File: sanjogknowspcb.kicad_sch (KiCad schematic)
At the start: 12 parts, among them SW1 SW_Push

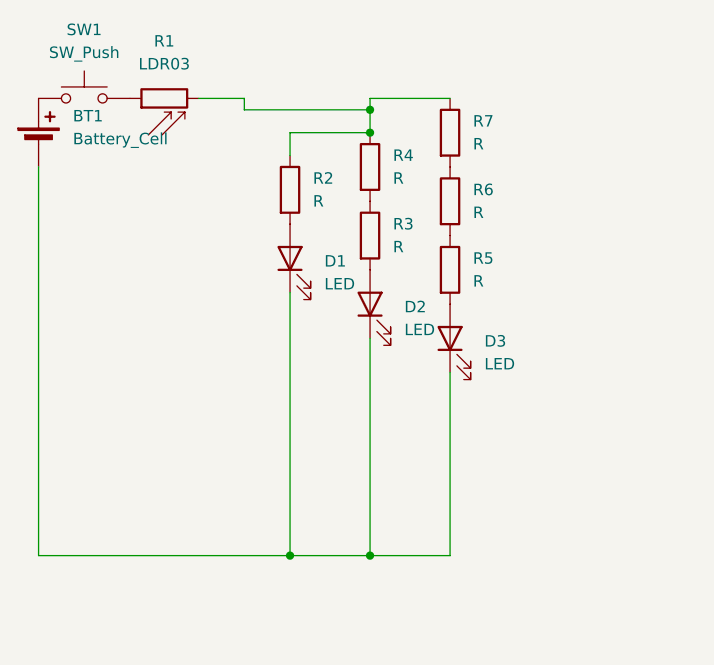
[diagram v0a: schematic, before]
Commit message: Add files via upload
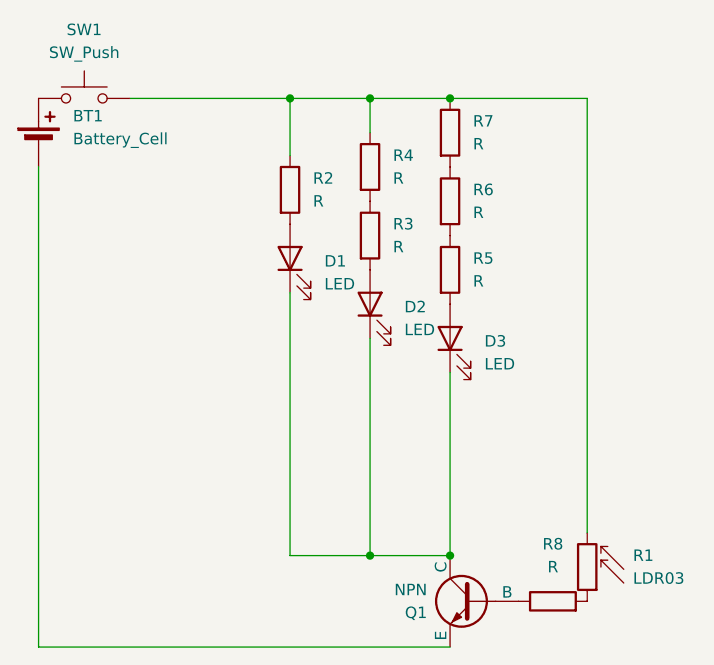
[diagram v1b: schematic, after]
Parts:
- added Q1: NPN, Package_TO_SOT_THT:TO-92L_HandSolder, symbol Simulation_SPICE:NPN
- added R8: R, Resistor_THT:R_Axial_DIN0207_L6.3mm_D2.5mm_P7.62mm_Horizontal, symbol Device:R
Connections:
- net at D1.1 (K), D2.1 (K), D3.1 (K): now also Q1.1 (C); no longer BT1.2 (-)
- net at R1.2, R2.1, R4.1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: now also SW1.2
- net at R1.1: now also R8.2; no longer SW1.2
- new net: Q1.2 (B), R8.1
- new net: BT1.2 (-), Q1.3 (E)
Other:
- moved on the sheet: R1
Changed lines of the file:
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@@
 	(paper "A4")
-	(junction
-		(at 66.04 124.46)
-		(diameter 0)
-		(color 0 0 0 0)
-	)
-	(junction
-		(at 74.93 77.47)
-		(diameter 0)
-		(color 0 0 0 0)
-	)
 	(junction
 		(at 74.93 124.46)
@@
 	)
 	(junction
-		(at 74.93 74.93)
+		(at 83.82 73.66)
 		(diameter 0)
 		(color 0 0 0 0)
 	)
-	(wire
-		(pts
-			(xy 66.04 80.01) (xy 66.04 77.47)
-		)
-		(stroke
-			(width 0)
-			(type default)
-		)
-	)
-	(wire
-		(pts
-			(xy 74.93 73.66) (xy 83.82 73.66)
-		)
-		(stroke
-			(width 0)
-			(type default)
-		)
-	)
-	(wire
-		(pts
-			(xy 74.93 77.47) (xy 74.93 74.93)
-		)
-		(stroke
-			(width 0)
-			(type default)
-		)
-	)
-	(wire
-		(pts
-			(xy 60.96 73.66) (xy 60.96 74.93)
-		)
-		(stroke
-			(width 0)
-			(type default)
-		)
-	)
-	(wire
-		(pts
-			(xy 74.93 74.93) (xy 60.96 74.93)
-		)
-		(stroke
-			(width 0)
-			(type default)
-		)
-	)
-	(wire
-		(pts
-			(xy 55.88 73.66) (xy 60.96 73.66)
-		)
-		(stroke
-			(width 0)
-			(type default)
-		)
-	)
-	(wire
-		(pts
-			(xy 38.1 124.46) (xy 38.1 81.28)
-		)
-		(stroke
-			(width 0)
-			(type default)
-		)
-	)
-	(wire
-		(pts
-			(xy 66.04 77.47) (xy 74.93 77.47)
-		)
-		(stroke
-			(width 0)
-			(type default)
-		)
-	)
-	(wire
-		(pts
-			(xy 74.93 74.93) (xy 74.93 73.66)
+	(junction
+		(at 66.04 73.66)
+		(diameter 0)
+		(color 0 0 0 0)
+	)
+	(junction
+		(at 83.82 124.46)
+		(diameter 0)
+		(color 0 0 0 0)
+	)
+	(junction
+		(at 74.93 73.66)
+		(diameter 0)
+		(color 0 0 0 0)
+	)
+	(wire
+		(pts
+			(xy 66.04 73.66) (xy 66.04 80.01)
+		)
+		(stroke
+			(width 0)
+			(type default)
+		)
+	)
+	(wire
+		(pts
+			(xy 74.93 73.66) (xy 74.93 77.47)
+		)
+		(stroke
+			(width 0)
+			(type default)
+		)
+	)
+	(wire
+		(pts
+			(xy 83.82 104.14) (xy 83.82 124.46)
+		)
+		(stroke
+			(width 0)
+			(type default)
+		)
+	)
+	(wire
+		(pts
+			(xy 99.06 73.66) (xy 83.82 73.66)
+		)
+		(stroke
+			(width 0)
+			(type default)
+		)
+	)
+	(wire
+		(pts
+			(xy 83.82 73.66) (xy 74.93 73.66)
+		)
+		(stroke
+			(width 0)
+			(type default)
+		)
+	)
+	(wire
+		(pts
+			(xy 99.06 121.92) (xy 99.06 73.66)
+		)
+		(stroke
+			(width 0)
+			(type default)
+		)
+	)
+	(wire
+		(pts
+			(xy 74.93 73.66) (xy 66.04 73.66)
+		)
+		(stroke
+			(width 0)
+			(type default)
+		)
+	)
+	(wire
+		(pts
+			(xy 83.82 134.62) (xy 38.1 134.62)
+		)
+		(stroke
+			(width 0)
+			(type default)
+		)
+	)
+	(wire
+		(pts
+			(xy 38.1 81.28) (xy 38.1 134.62)
 		)
 		(stroke
@@
 	(wire
 		(pts
-			(xy 38.1 124.46) (xy 66.04 124.46)
-		)
-		(stroke
-			(width 0)
-			(type default)
-		)
-	)
-	(wire
-		(pts
 			(xy 74.93 100.33) (xy 74.93 124.46)
 		)
@@
 	(wire
 		(pts
-			(xy 83.82 104.14) (xy 83.82 124.46)
-		)
-		(stroke
-			(width 0)
-			(type default)
-		)
-	)
-	(wire
-		(pts
 			(xy 66.04 124.46) (xy 74.93 124.46)
 		)
@@
 		(pts
 			(xy 74.93 124.46) (xy 83.82 124.46)
+		)
+		(stroke
+			(width 0)
+			(type default)
+		)
+	)
+	(wire
+		(pts
+			(xy 66.04 73.66) (xy 48.26 73.66)
 		)
 		(stroke
@@
 	)
 	(symbol
+		(lib_id "Simulation_SPICE:NPN")
+		(at 86.36 129.54 0)
+		(mirror y)
+		(unit 1)
+		(exclude_from_sim no)
+		(in_bom yes)
+		(on_board yes)
+		(dnp no)
+		(property "Reference" "Q1"
+			(at 81.28 130.8101 0)
+			(effects
+				(font
+					(size 1.27 1.27)
+				)
+				(justify left)
+			)
+		)
+		(property "Value" "NPN"
+			(at 81.28 128.2701 0)
+			(effects
+				(font
+					(size 1.27 1.27)
+				)
+				(justify left)
+			)
+		)
+		(property "Footprint" "Package_TO_SOT_THT:TO-92L_HandSolder"
+			(at 22.86 129.54 0)
+			(effects
+				(font
+					(size 1.27 1.27)
+				)
+				(hide yes)
+			)
+		)
+		(property "Datasheet" "https://ngspice.sourceforge.io/docs/ngspice-html-manual/manual.xhtml#cha_BJTs"
+			(at 22.86 129.54 0)
+			(effects
+				(font
+					(size 1.27 1.27)
+				)
+				(hide yes)
+			)
+		)
+		(property "Description" "Bipolar transistor symbol for simulation only, substrate tied to the emitter"
+			(at 86.36 129.54 0)
+			(effects
+				(font
+					(size 1.27 1.27)
+				)
+				(hide yes)
+			)
+		)
+		(property "Sim.Device" "NPN"
+			(at 86.36 129.54 0)
+			(effects
+				(font
+					(size 1.27 1.27)
+				)
+				(hide yes)
+			)
+		)
+		(property "Sim.Type" "GUMMELPOON"
+			(at 86.36 129.54 0)
+			(effects
+				(font
+					(size 1.27 1.27)
+				)
+				(hide yes)
+			)
+		)
+		(property "Sim.Pins" "1=C 2=B 3=E"
+			(at 86.36 129.54 0)
+			(effects
+				(font
+					(size 1.27 1.27)
+				)
+				(hide yes)
+			)
+		)
+		(pin "3"
+		)
+		(pin "1"
+		)
+		(pin "2"
+		)
+		(instances
+			(project ""
+				(path "/80278f69-b966-473c-8055-8c9a8f6f86ca"
+					(reference "Q1")
+					(unit 1)
+				)
+			)
+		)
+	)
+	(symbol
 		(lib_id "Device:Battery_Cell")
 		(at 38.1 78.74 0)
@@
 	(symbol
 		(lib_id "Sensor_Optical:LDR03")
-		(at 52.07 73.66 90)
+		(at 99.06 125.73 180)
 		(unit 1)
 		(exclude_from_sim no)
@@
 		(fields_autoplaced yes)
 		(property "Reference" "R1"
-			(at 52.07 67.31 90)
-			(effects
-				(font
-					(size 1.27 1.27)
-				)
+			(at 104.14 124.4599 0)
+			(effects
+				(font
+					(size 1.27 1.27)
+				)
+				(justify right)
 			)
 		)
 		(property "Value" "LDR03"
-			(at 52.07 69.85 90)
-			(effects
-				(font
-					(size 1.27 1.27)
-				)
+			(at 104.14 126.9999 0)
+			(effects
+				(font
+					(size 1.27 1.27)
+				)
+				(justify right)
 			)
 		)
 		(property "Footprint" "OptoDevice:R_LDR_5.1x4.3mm_P3.4mm_Vertical"
-			(at 52.07 69.215 90)
+			(at 94.615 125.73 90)
 			(effects
 				(font
@@
 		)
 		(property "Datasheet" "http://www.elektronica-componenten.nl/WebRoot/StoreNL/Shops/61422969/54F1/BA0C/C664/31B9/2173/C0A8/2AB9/2AEF/LDR03IMP.pdf"
-			(at 53.34 73.66 0)
+			(at 99.06 124.46 0)
 			(effects
 				(font
@@
 		)
 		(property "Description" "light dependent resistor"
-			(at 52.07 73.66 0)
+			(at 99.06 125.73 0)
 			(effects
 				(font
@@
 					(unit 1)
 				)
+			)
+		)
+	)
+	(symbol
+		(lib_id "Device:R")
+		(at 95.25 129.54 90)
+		(unit 1)
+		(exclude_from_sim no)
+		(in_bom yes)
+		(on_board yes)
+		(dnp no)
+		(fields_autoplaced yes)
+		(property "Reference" "R8"
+			(at 95.25 123.19 90)
+			(effects
+				(font
+					(size 1.27 1.27)
+				)
+			)
+		)
+		(property "Value" "R"
+			(at 95.25 125.73 90)
+			(effects
+				(font
+					(size 1.27 1.27)
+				)
+			)
+		)
+		(property "Footprint" "Resistor_THT:R_Axial_DIN0207_L6.3mm_D2.5mm_P7.62mm_Horizontal"
+			(at 95.25 131.318 90)
+			(effects
+				(font
+					(size 1.27 1.27)
+				)
+				(hide yes)
+			)
+		)
+		(property "Datasheet" "~"
+			(at 95.25 129.54 0)
+			(effects
+				(font
+					(size 1.27 1.27)
+				)
+				(hide yes)
+			)
+		)
+		(property "Description" "Resistor"
+			(at 95.25 129.54 0)
+			(effects
+				(font
+					(size 1.27 1.27)
+				)
+				(hide yes)
+			)
+		)
+		(pin "2"
+		)
+		(pin "1"
+		)
+		(instances
+			(project ""
+				(path "/80278f69-b966-473c-8055-8c9a8f6f86ca"
+					(reference "R8")
+					(unit 1)
+				)
